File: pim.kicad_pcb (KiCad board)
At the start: 2 copper layers, 96.4 x 66.5 mm, 13 parts, among them J1 DE9_Plug, J2 DE9_Plug, J3 Conn_01x20_Pin, J4 Conn_01x03_MountingPin, U1 RaspberryPi_Pico_W

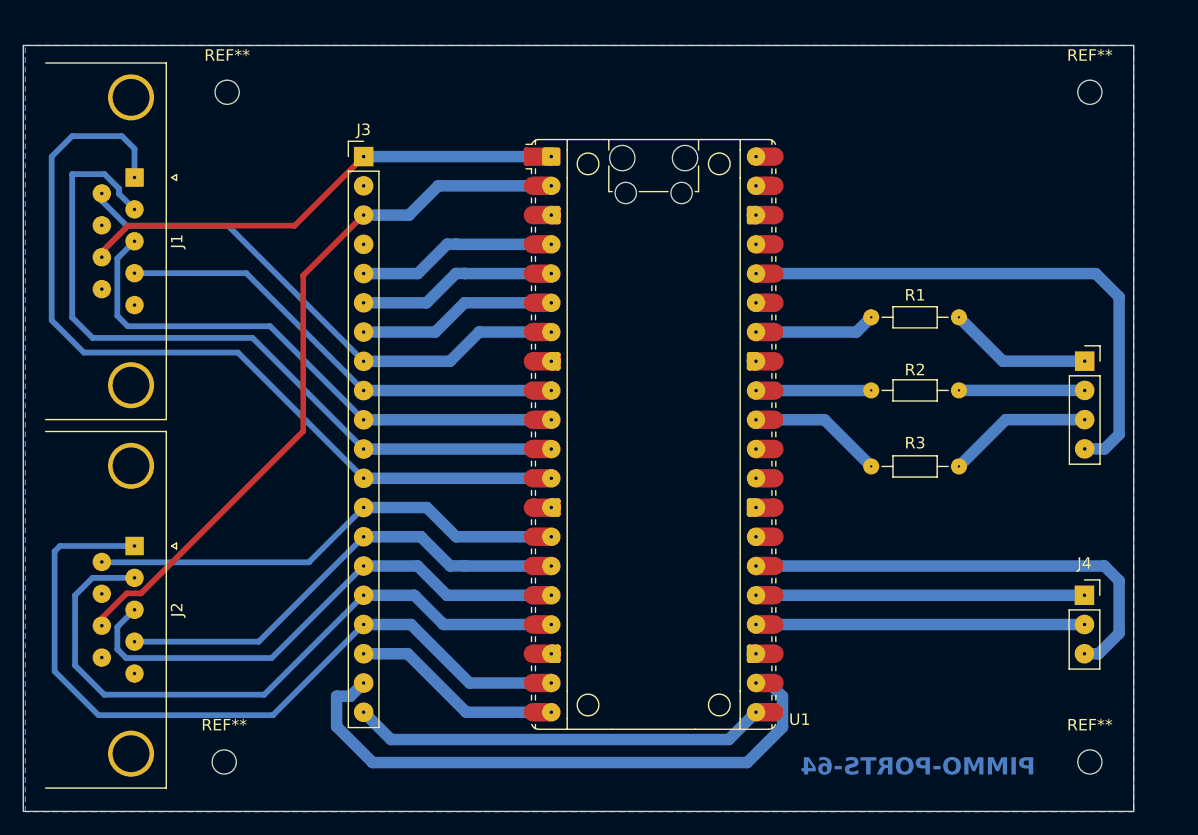
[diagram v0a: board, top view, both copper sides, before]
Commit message: Some minor improvements
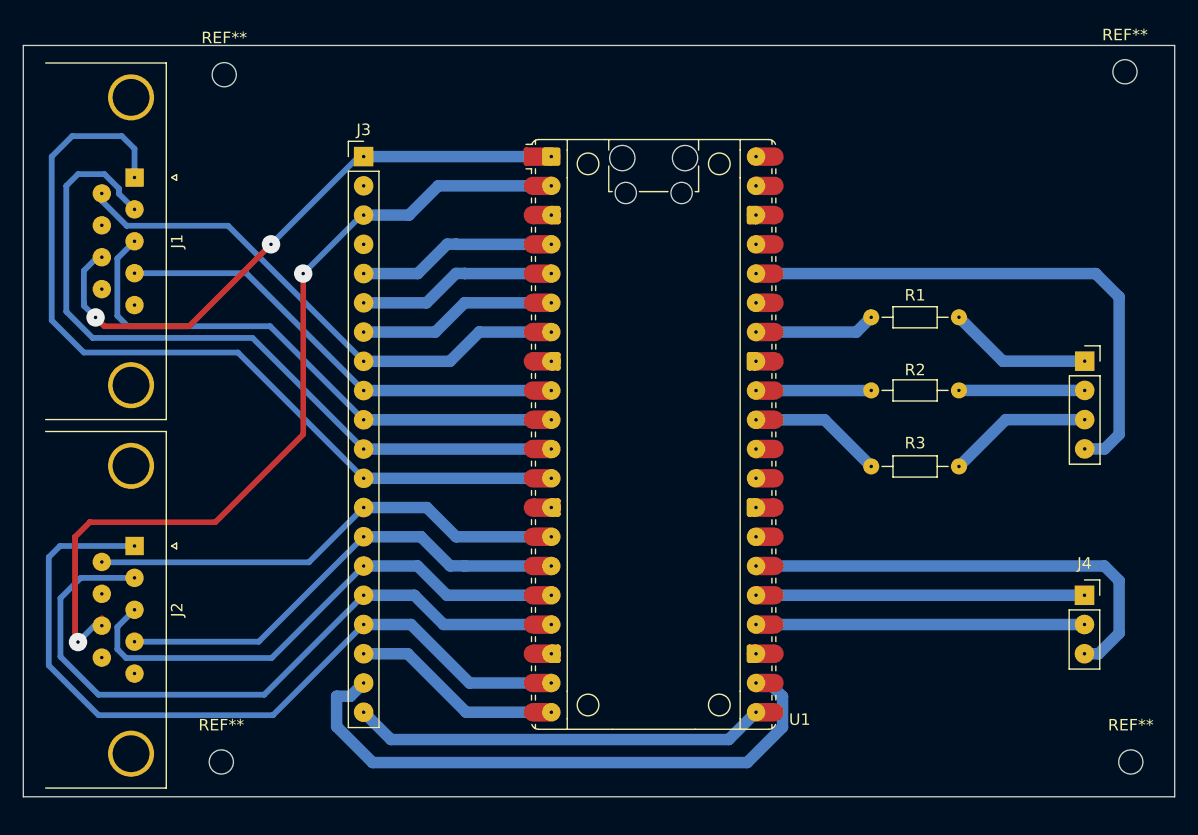
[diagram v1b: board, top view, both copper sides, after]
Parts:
- moved REF** 3.56 mm to (116.1, 76.2)
- moved REF** 3.53 mm to (115.6, 16.3)
- moved REF** 1.55 mm to (37.3, 16.5)
- moved REF** 0.25 mm to (37.1, 76.2)
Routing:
- net /M-8: track 63.2 -> 75.1 mm, vias 0 -> 2
- net /M-i: track 42.9 -> 52.6 mm, vias 0 -> 2
- net /M-e: track 58.9 -> 60.9 mm
- removed copper zone on B.Cu, net GNDPWR
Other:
- board size 96.4 x 66.5 mm -> 100 x 65.3 mm
